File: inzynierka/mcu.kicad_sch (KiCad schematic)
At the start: 23 parts, among them J4 Conn_01x04_Socket, U6 nRF52840, Y2 32.786k

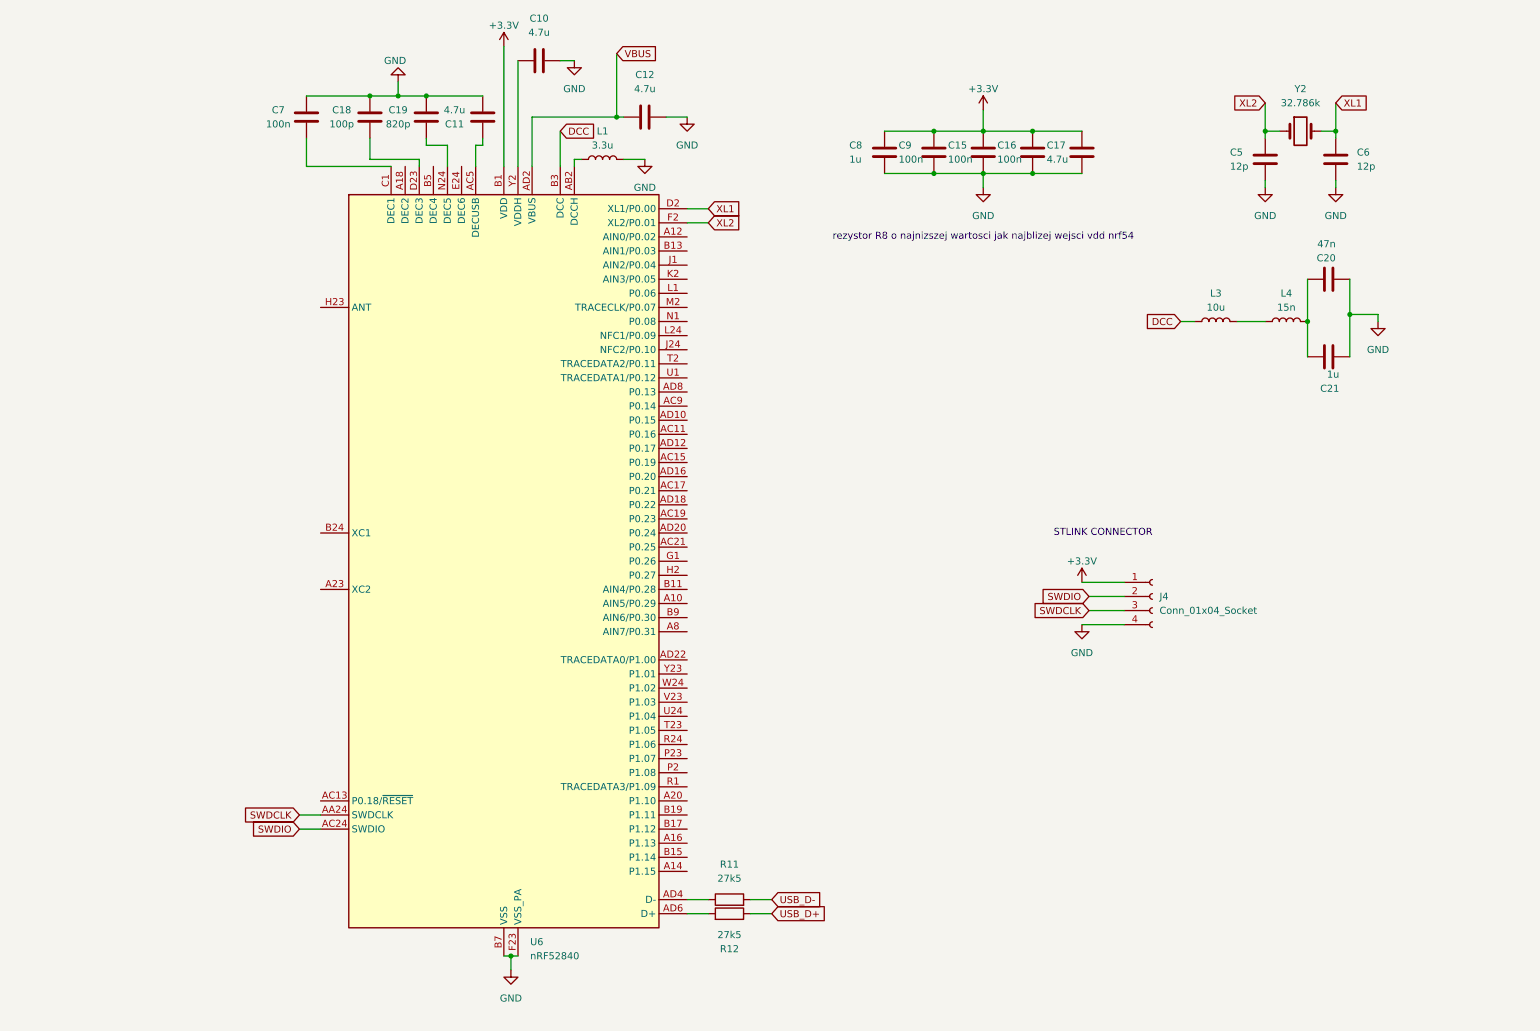
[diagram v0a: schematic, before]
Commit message: Add files via upload
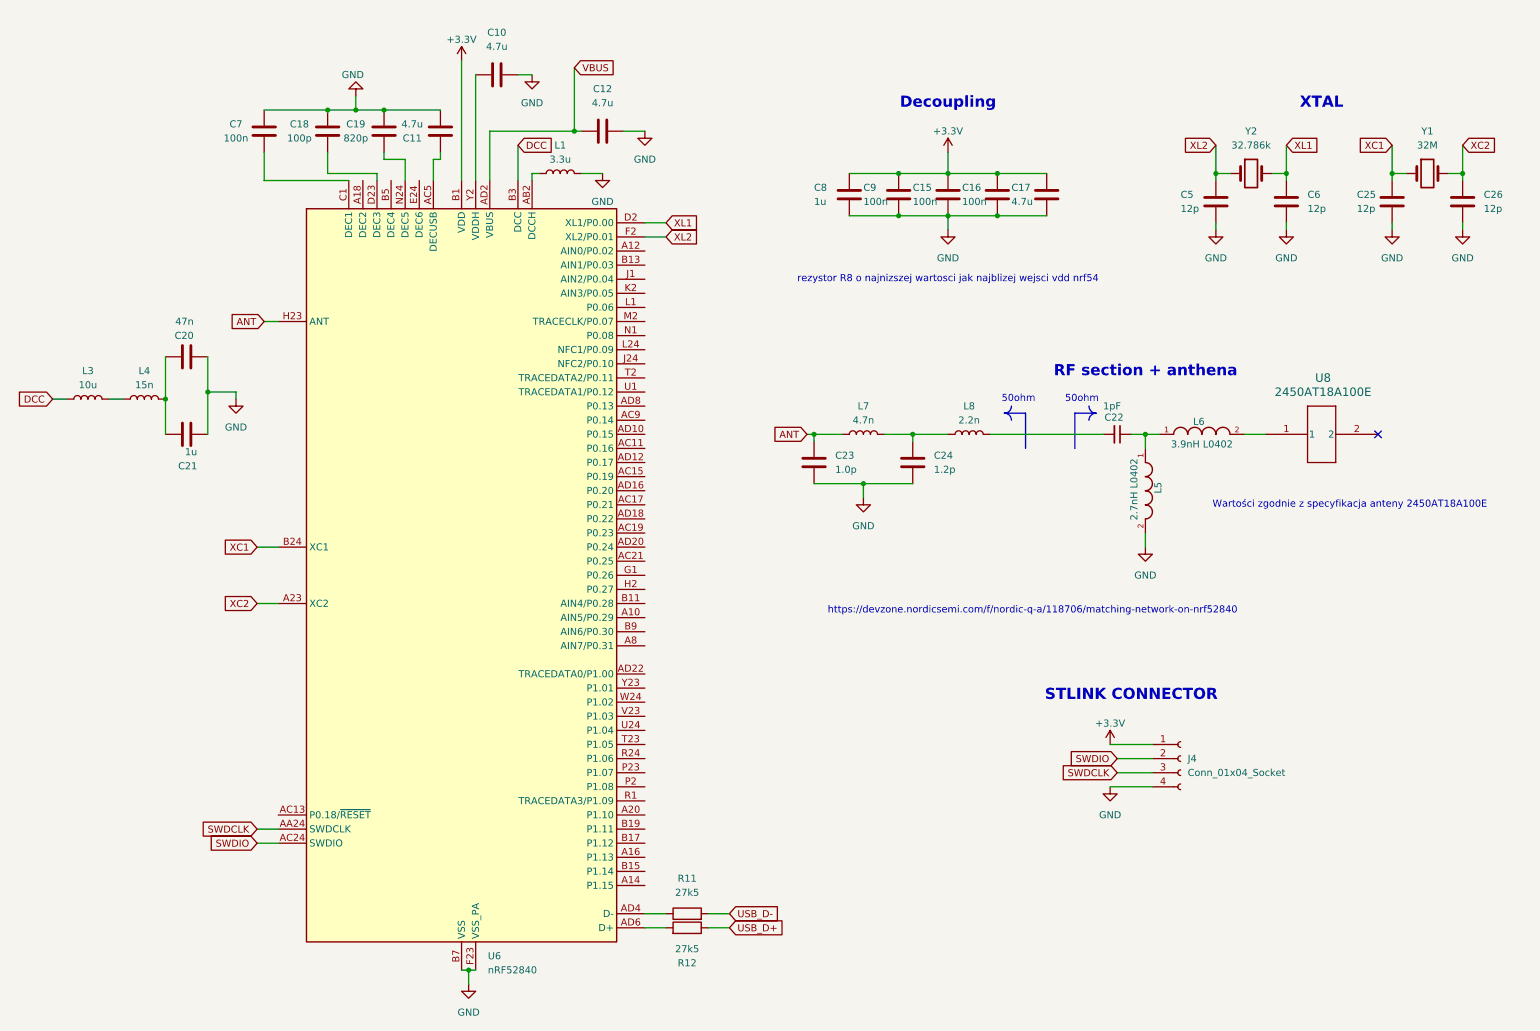
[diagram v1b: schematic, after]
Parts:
- added C22: 1pF, Capacitor_SMD:C_0402_1005Metric, symbol Device:C_Small
- added C23: 1.0p, symbol Device:C
- added C24: 1.2p, symbol Device:C
- added C25, C26: 12p, symbol Device:C
- added L5: 2.7nH L0402, Inductor_SMD:L_0402_1005Metric, symbol DFE201612E-2R2M_P2:DFE201612E-2R2M=P2
- added L6: 3.9nH L0402, Inductor_SMD:L_0402_1005Metric, symbol DFE201612E-2R2M_P2:DFE201612E-2R2M=P2
- added L7: 4.7n, symbol Device:L
- added L8: 2.2n, symbol Device:L
- added U8: 2450AT18A100E, RF_Antenna:Johanson_2450AT18x100, symbol 2450AT18A0100001E:2450AT18A100E
- added Y1: 32M, symbol Device:Crystal
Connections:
- net GND: now also C23.2, C24.2, C25.2, C26.2, L5.2
- net XC2: now reaches U6.A23 (XC2)
- net XC2: now also C26.1, Y1.2
- net XC1: now reaches U6.B24 (XC1)
- net XC1: now also C25.1, Y1.1
- net ANT: now reaches U6.H23 (ANT)
- net ANT: now also C23.1, L7.1
- new net: C24.1, L7.2, L8.1
- new net: C22.2, L8.2
- new net: C22.1, L5.1, L6.1
- new net: L6.2, U8.1
- no-connect marks 0 -> 1
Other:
- note added: "50ohm"
- note added: "Decoupling"
- note added: "RF section + anthena"
- note added: "Wartości zgodnie z specyfikacja anteny 2450AT18A100E"
- note added: "XTAL"
- note added: "https://devzone.nordicsemi.com/f/nordic-q-a/118706/matching-network-on-nrf52840"
- moved on the sheet: C10, C11, C12, C15, C16, C17, C18, C19, C20, C21, C5, C6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
